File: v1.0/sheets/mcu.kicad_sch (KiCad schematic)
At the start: 18 parts, among them IC1 STM32U5G7VJT6Q

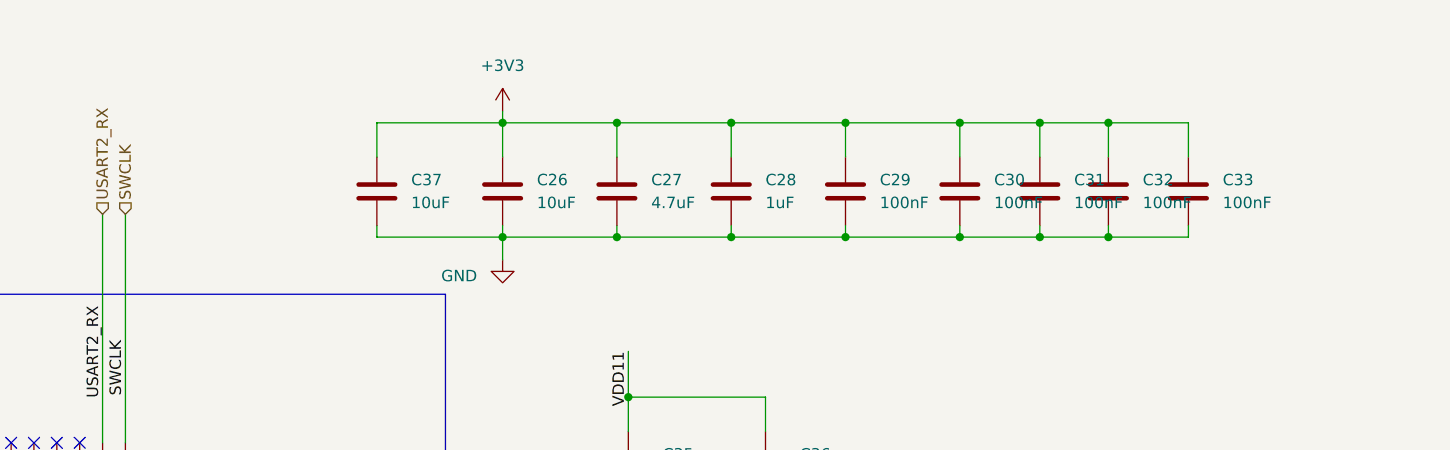
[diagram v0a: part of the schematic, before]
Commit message: Revision V2.0 finalized
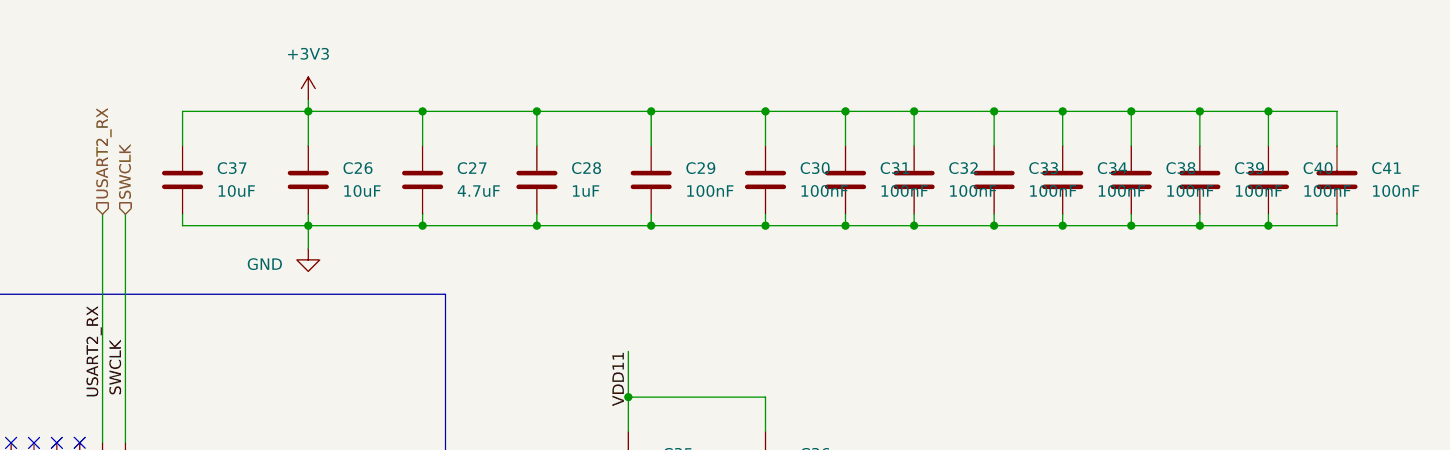
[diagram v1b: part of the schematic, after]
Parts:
- added C34, C38, C39, C40, C41: 100nF, Capacitor_SMD:C_0402_1005Metric, symbol Device:C
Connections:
- net +3V3: now also C34.2, C38.2, C39.2, C40.2, C41.2
- net GND: now also C34.1, C38.1, C39.1, C40.1, C41.1
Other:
- moved on the sheet: C26, C27, C28, C29, C30, C31, C32, C33, C37
